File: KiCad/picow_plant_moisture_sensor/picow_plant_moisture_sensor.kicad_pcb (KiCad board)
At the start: 4 copper layers, 74 x 52 mm, 52 parts, among them J2 AudioJack3, J3 Micro_SD_Card, J4 L77HDE15SD1CH4F, J7 Conn_02x03_Odd_Even, SW1 SW_Push, SW2 SW_Push, SW3 SW_Push, SW4 SW_Push, U1 TLV70033_SOT23-5, U2 PicoW, U3 NC7WZ16P6X

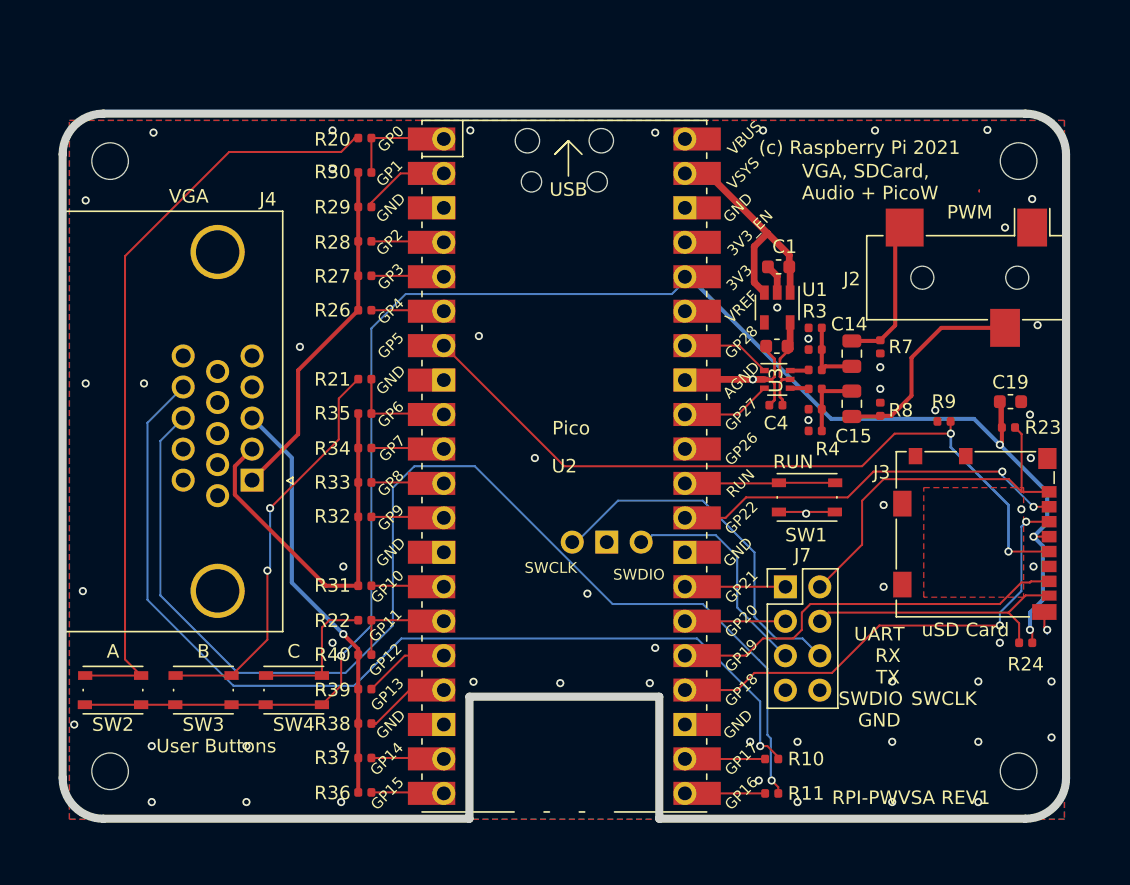
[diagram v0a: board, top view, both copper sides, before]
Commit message: First version done
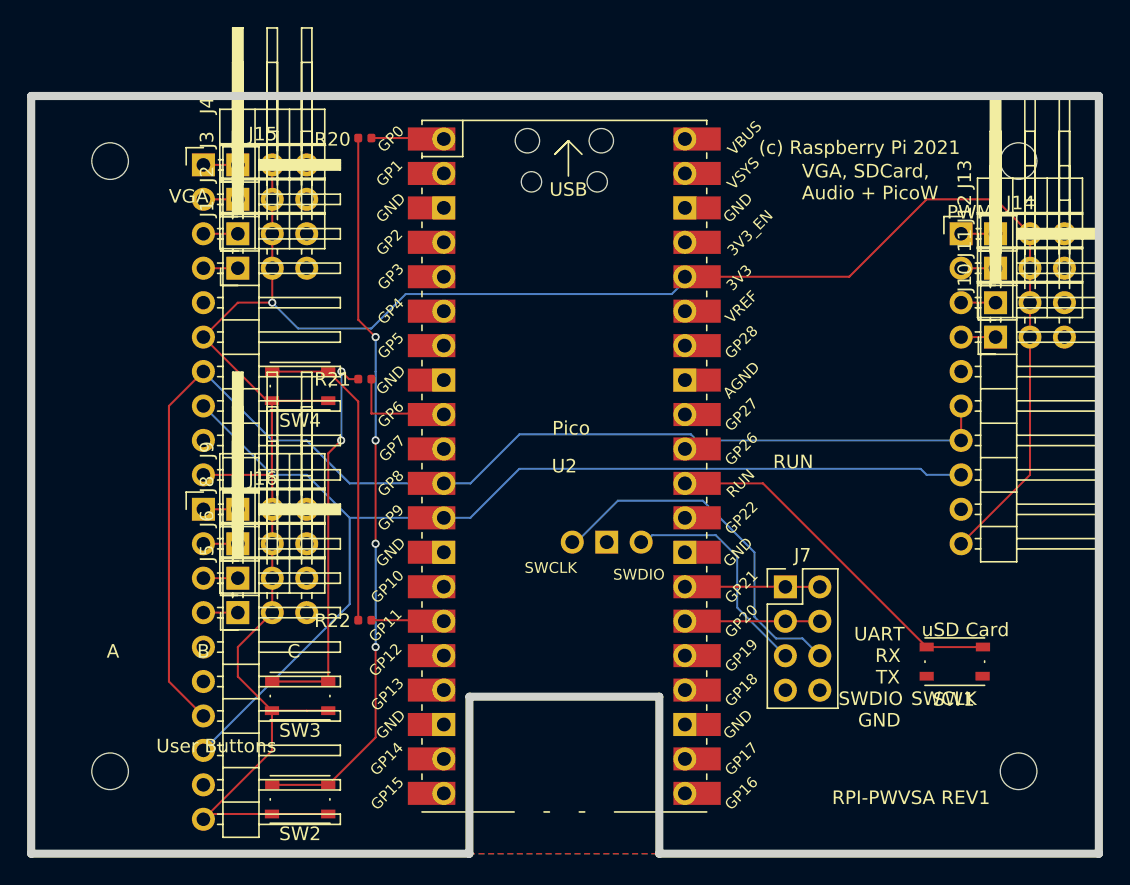
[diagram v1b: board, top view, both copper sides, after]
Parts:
- removed C1, C2: 1u, Capacitor_SMD:C_0603_1608Metric
- removed C14, C15: 47u, Capacitor_SMD:C_0805_2012Metric
- removed C19: 10u, Capacitor_SMD:C_0603_1608Metric
- removed C4, C7, C8: 100n, Capacitor_SMD:C_0402_1005Metric
- removed R1, R2: 220, Resistor_SMD:R_0402_1005Metric
- removed R10, R11: 47, Resistor_SMD:R_0402_1005Metric
- removed R23, R24: 10k, Resistor_SMD:R_0402_1005Metric
- removed R26, R31, R36: 499, Resistor_SMD:R_0402_1005Metric
- removed R27, R32, R37: 1k, Resistor_SMD:R_0402_1005Metric
- removed R28, R33, R38: 2k, Resistor_SMD:R_0402_1005Metric
- removed R29, R34, R39: 4.02k, Resistor_SMD:R_0402_1005Metric
- removed R3, R4: 100, Resistor_SMD:R_0402_1005Metric
- removed R30, R35, R40: 8.06k, Resistor_SMD:R_0402_1005Metric
- removed R7, R8: 1.8K, Resistor_SMD:R_0402_1005Metric
- removed R9: DNF, Resistor_SMD:R_0402_1005Metric
- removed U1: TLV70033_SOT23-5, Package_TO_SOT_SMD:SOT-23-5
- removed U3: NC7WZ16P6X, Package_TO_SOT_SMD:SOT-363_SC-70-6
- added J1: Conn_01x03, Connector_PinHeader_2.54mm:PinHeader_1x03_P2.54mm_Horizontal, F.Cu at (106.4, 60.4)
- added J10: Conn_01x03, Connector_PinHeader_2.54mm:PinHeader_1x03_P2.54mm_Horizontal, F.Cu at (162.3, 65.5)
- added J11: Conn_01x03, Connector_PinHeader_2.54mm:PinHeader_1x03_P2.54mm_Horizontal, F.Cu at (162.3, 62.9)
- added J12: Conn_01x03, Connector_PinHeader_2.54mm:PinHeader_1x03_P2.54mm_Horizontal, F.Cu at (162.3, 60.4)
- added J13: Conn_01x03, Connector_PinHeader_2.54mm:PinHeader_1x03_P2.54mm_Horizontal, F.Cu at (162.3, 57.9)
- added J14: ADS1115, Connector_PinHeader_2.54mm:PinHeader_1x10_P2.54mm_Horizontal, F.Cu at (159.8, 57.9)
- added J15: ADS1115, Connector_PinHeader_2.54mm:PinHeader_1x10_P2.54mm_Horizontal, F.Cu at (103.9, 52.8)
- added J16: ADS1115, Connector_PinHeader_2.54mm:PinHeader_1x10_P2.54mm_Horizontal, F.Cu at (103.9, 78.2)
- added J5: Conn_01x03, Connector_PinHeader_2.54mm:PinHeader_1x03_P2.54mm_Horizontal, F.Cu at (106.4, 85.8)
- added J6: Conn_01x03, Connector_PinHeader_2.54mm:PinHeader_1x03_P2.54mm_Horizontal, F.Cu at (106.4, 83.3)
- added J8: Conn_01x03, Connector_PinHeader_2.54mm:PinHeader_1x03_P2.54mm_Horizontal, F.Cu at (106.4, 80.7)
- added J9: Conn_01x03, Connector_PinHeader_2.54mm:PinHeader_1x03_P2.54mm_Horizontal, F.Cu at (106.4, 78.2)
- J2: value AudioJack3 -> Conn_01x03; footprint RPi_Pico:CUI_SJ-3523-audio-jack -> Connector_PinHeader_2.54mm:PinHeader_1x03_P2.54mm_Horizontal
- J3: value Micro_SD_Card -> Conn_01x03; footprint Connector_Card:microSD_HC_Molex_104031-0811 -> Connector_PinHeader_2.54mm:PinHeader_1x03_P2.54mm_Horizontal
- J4: value L77HDE15SD1CH4F -> Conn_01x03; footprint RPi_Pico:DSUB-15-L77HDE15SD1CH4F -> Connector_PinHeader_2.54mm:PinHeader_1x03_P2.54mm_Horizontal
- moved J3 59.7 mm to (106.4, 55.3), turned to 90 degrees
- moved J2 55.1 mm to (106.4, 57.9), turned to 90 degrees
- moved J4 22.9 mm to (106.4, 52.8)
- moved SW4 22.4 mm to (111.0, 69.1)
- moved SW1 16.3 mm to (159.3, 89.4)
- moved SW2 16.0 mm to (111.0, 99.6)
- moved SW3 7.14 mm to (111.0, 92.0)
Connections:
- J2 pad 1: GND -> /AIN5
- J2 pad 2: /PWM_AUDIO_L -> +3V3
- J2 pad 3: /PWM_AUDIO_R -> GND
- J3 pad 1: /SD_DAT2 -> /AIN6
- J3 pad 2: /GPIO22 -> +3V3
- J3 pad 3: /GPIO18 -> GND
- J4 pad 1: /VGA_R -> /AIN7
- J4 pad 2: /VGA_G -> +3V3
- J4 pad 3: /VGA_B -> GND
- J7 pad 2: /SD_DAT2 -> /GPIO21
- J7 pad 4: /SD_DAT1 -> /GPIO20
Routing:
- net /HSYNC: track 89.2 -> 0.00 mm, vias 1 -> 0
- net /GPIO8: track 5.37 -> 91.0 mm
- net /GPIO9: track 5.37 -> 82.6 mm
- net /VSYNC: track 73.1 -> 0.00 mm, vias 1 -> 0
- net /GPIO5: track 56.4 -> 0.00 mm, vias 2 -> 0
- net +3V3: track 123.4 -> 173.4 mm, vias 4 -> 1
- net /GPIO18: track 35.4 -> 0.00 mm, vias 2 -> 0
- net /VGA_B: track 30.9 -> 0.00 mm, vias 1 -> 0
- net /GPIO19: track 29.9 -> 0.00 mm
- net /GPIO22: track 29.7 -> 0.00 mm, vias 2 -> 0
- net /VGA_G: track 28.5 -> 0.00 mm
- net /SD_DAT2: track 27.4 -> 0.00 mm
- net /VGA_R: track 25.9 -> 0.00 mm
- net GND: track 25.0 -> 0.00 mm, vias 60 -> 0
- net /SD_DAT1: track 20.3 -> 0.00 mm
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- removed copper zone on In1.Cu, net GND
- removed copper zone on In2.Cu, net GND
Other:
- board size 74 x 52 mm -> 78.7 x 55.9 mm
- copper layers 4 -> 2

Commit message: V1 done
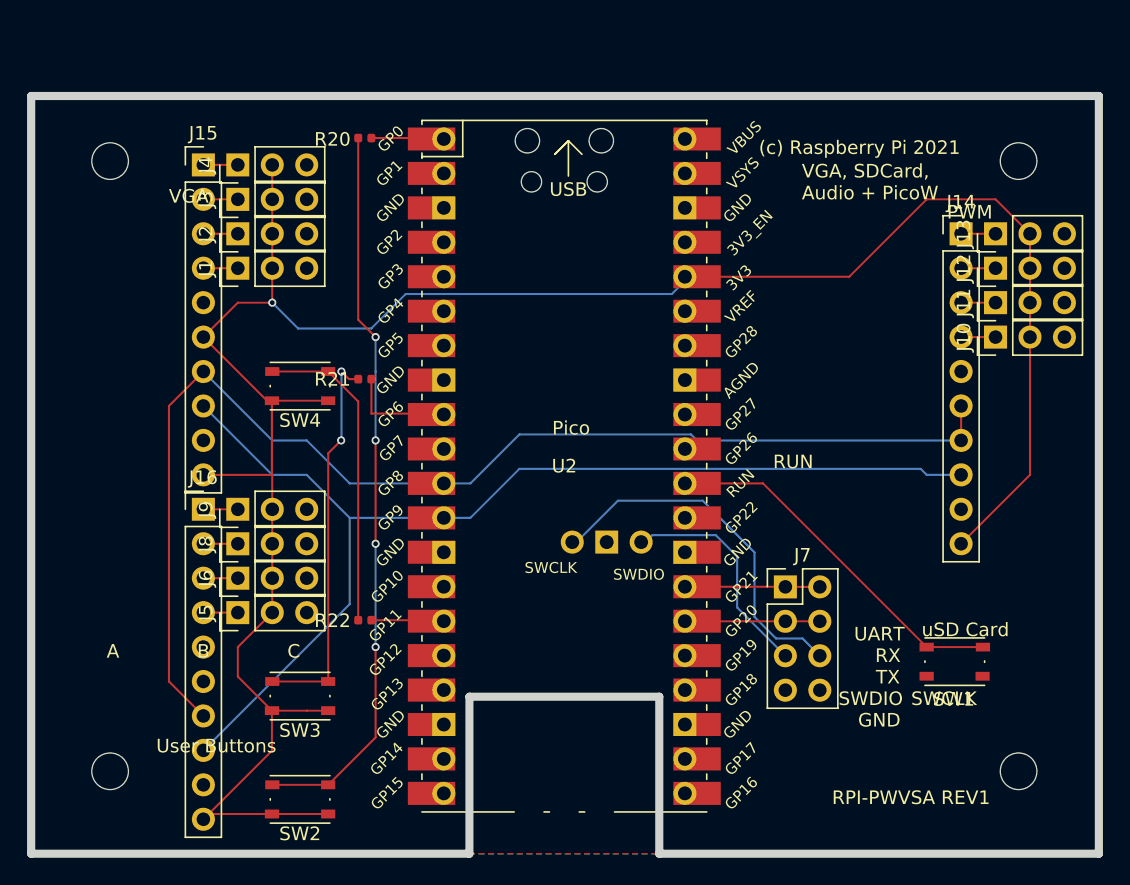
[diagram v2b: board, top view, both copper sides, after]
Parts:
- J1, J10, J11, J12, J13, J2, J3, J4, J5, J6, J8, J9: footprint Connector_PinHeader_2.54mm:PinHeader_1x03_P2.54mm_Horizontal -> Connector_PinHeader_2.54mm:PinHeader_1x03_P2.54mm_Vertical
- J14, J15, J16: footprint Connector_PinHeader_2.54mm:PinHeader_1x10_P2.54mm_Horizontal -> Connector_PinHeader_2.54mm:PinHeader_1x10_P2.54mm_Vertical
